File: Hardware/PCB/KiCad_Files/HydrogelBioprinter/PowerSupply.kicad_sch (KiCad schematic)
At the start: 11 parts, among them J3 Screw_Terminal_01x02, U4 AP3211KTR-G1

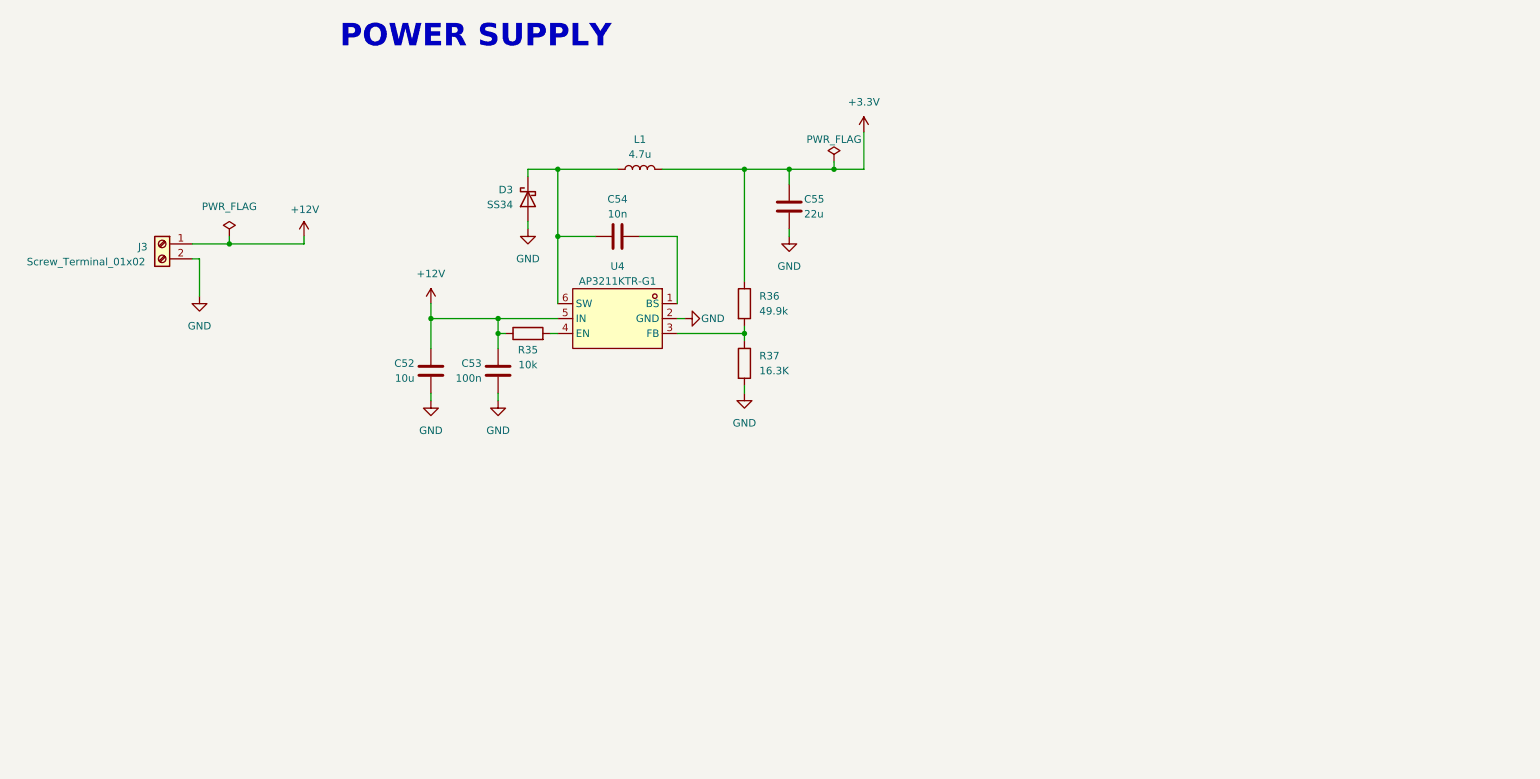
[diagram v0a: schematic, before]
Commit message: Schematic Update, PCB preliminary layout, Machine Design addition, and LaTeX report addition
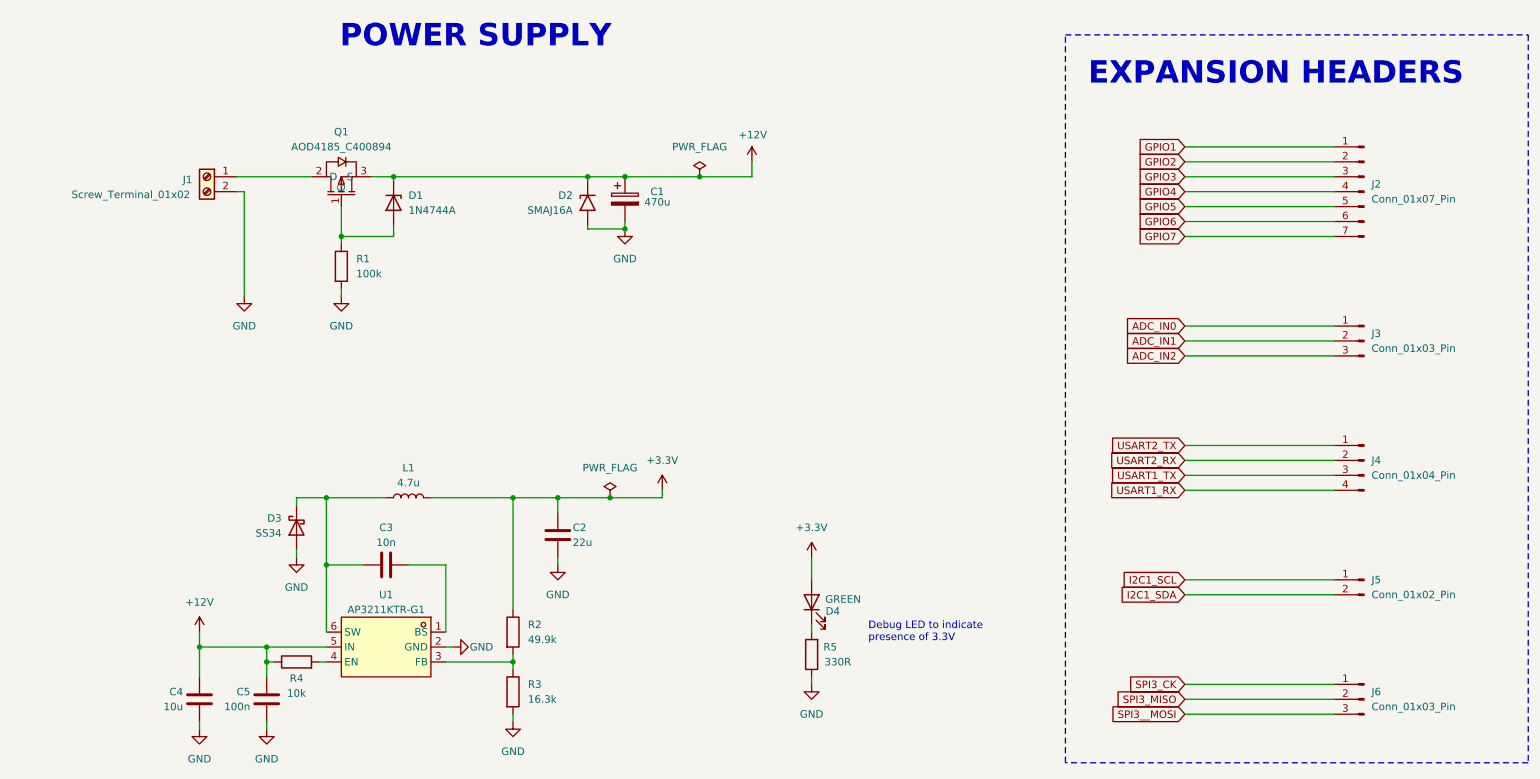
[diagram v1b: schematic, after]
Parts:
- added C1: 470u, Capacitor_THT:CP_Radial_D10.0mm_P5.00mm, symbol Device:C_Polarized
- added D1: 1N4744A, Diode_THT:D_DO-41_SOD81_P10.16mm_Horizontal, symbol Diode:1N47xxA
- added D2: SMAJ16A, Diode_SMD:D_SMA, symbol Diode:SMAJ16A
- added D4: GREEN, LED_SMD:LED_0805_2012Metric, symbol Device:LED
- added J2: Conn_01x07_Pin, Connector_PinHeader_2.54mm:PinHeader_1x07_P2.54mm_Vertical, symbol Connector:Conn_01x07_Pin
- added J3, J6: Conn_01x03_Pin, Connector_PinHeader_2.54mm:PinHeader_1x03_P2.54mm_Vertical, symbol Connector:Conn_01x03_Pin
- added J4: Conn_01x04_Pin, Connector_PinHeader_2.54mm:PinHeader_1x04_P2.54mm_Vertical, symbol Connector:Conn_01x04_Pin
- added J5: Conn_01x02_Pin, Connector_PinHeader_2.54mm:PinHeader_1x02_P2.54mm_Vertical, symbol Connector:Conn_01x02_Pin
- added Q1: AOD4185_C400894, AOD4185:TO-252-3_L6.6-W6.1-P4.57-LS9.9-BR-CW, symbol AOD4185:AOD4185_C400894
- added R1: 100k, Resistor_SMD:R_0805_2012Metric, symbol Device:R
- added R5: 330R, Resistor_THT:R_Axial_DIN0207_L6.3mm_D2.5mm_P10.16mm_Horizontal, symbol Device:R
- C2: renamed from C55; footprint (none) -> Capacitor_SMD:C_0805_2012Metric
- C3: renamed from C54; footprint (none) -> Capacitor_SMD:C_0603_1608Metric
- C4: renamed from C52; footprint (none) -> Capacitor_SMD:C_0805_2012Metric
- C5: renamed from C53; footprint (none) -> Capacitor_SMD:C_0603_1608Metric
- J1: renamed from J3; footprint (none) -> TerminalBlock_Phoenix:TerminalBlock_Phoenix_MKDS-1,5-2-5.08_1x02_P5.08mm_Horizontal
- L1: footprint (none) -> Inductor_SMD:L_7.3x7.3_H4.5
- R2: renamed from R36; footprint (none) -> Resistor_THT:R_Axial_DIN0207_L6.3mm_D2.5mm_P10.16mm_Horizontal
- R3: renamed from R37; value 16.3K -> 16.3k; footprint (none) -> Resistor_THT:R_Axial_DIN0207_L6.3mm_D2.5mm_P10.16mm_Horizontal
- R4: renamed from R35; footprint (none) -> Resistor_SMD:R_0805_2012Metric
- U1: renamed from U4; footprint easyeda2kicad:SOT-23-6_L2.9-W1.6-P0.95-LS2.8-BR -> AP3211KTR-G1:AP3211KTR-G1
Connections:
- net +12V: now also C1.1, D1.1 (K), D2.1 (A1), Q1.3 (S); no longer J1.1 (Pin_1)
- net +3.3V: now also D4.2 (A)
- net GND: now also C1.2, D2.2 (A2), R1.2, R5.1
- new net: D1.2 (A), Q1.1 (G), R1.1
- new net: J1.1 (Pin_1), Q1.2 (D)
- new net: D4.1 (K), R5.2
- new net ADC_IN0: J3.1 (Pin_1)
- new net ADC_IN1: J3.2 (Pin_2)
- new net ADC_IN2: J3.3 (Pin_3)
- new net GPIO1: J2.1 (Pin_1)
- new net GPIO2: J2.2 (Pin_2)
- new net GPIO3: J2.3 (Pin_3)
- new net GPIO4: J2.4 (Pin_4)
- new net GPIO5: J2.5 (Pin_5)
- new net GPIO6: J2.6 (Pin_6)
- new net GPIO7: J2.7 (Pin_7)
- new net I2C1_SCL: J5.1 (Pin_1)
- new net I2C1_SDA: J5.2 (Pin_2)
- new net SPI3_CK: J6.1 (Pin_1)
- new net SPI3_MISO: J6.2 (Pin_2)
- new net SPI3__MOSI: J6.3 (Pin_3)
- new net USART1_RX: J4.4 (Pin_4)
- new net USART1_TX: J4.3 (Pin_3)
- new net USART2_RX: J4.2 (Pin_2)
- new net USART2_TX: J4.1 (Pin_1)
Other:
- note added: "Debug LED to indicate presence of 3.3V"
- note added: "EXPANSION HEADERS"
- moved on the sheet: C2, C3, C4, C5, D3, J1, L1, R2, R3, R4, U1

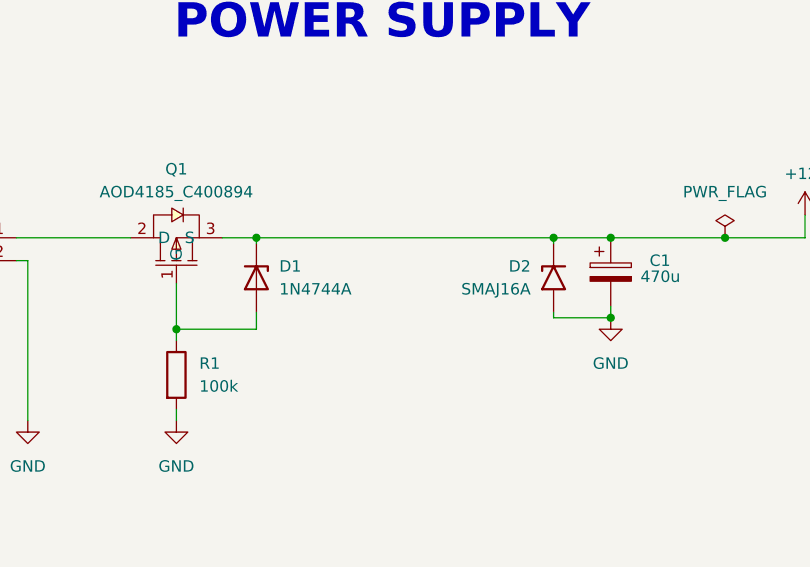
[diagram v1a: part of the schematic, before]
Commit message: Gantry Concept 1 Completion and PCB schematic update
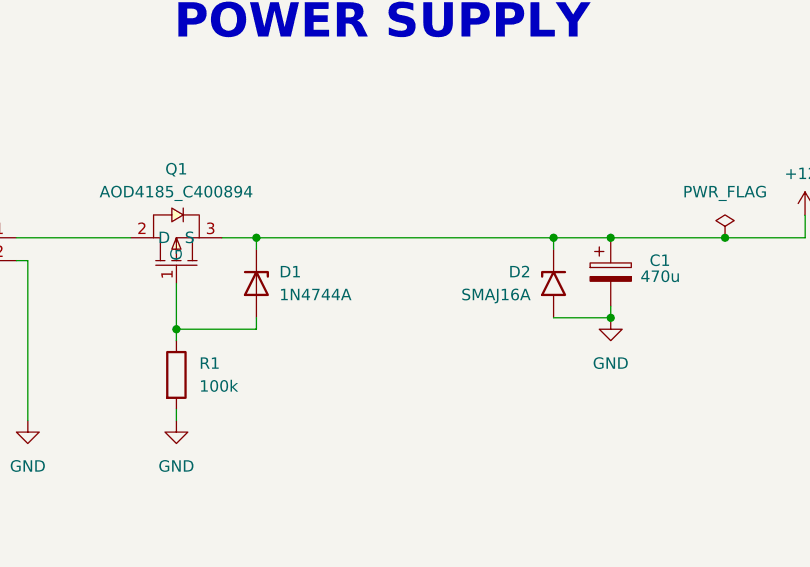
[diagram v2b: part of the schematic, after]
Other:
- moved on the sheet: D1, D2
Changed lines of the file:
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@@
 	)
 	(junction
+		(at 82.55 57.15)
+		(diameter 0)
+		(color 0 0 0 0)
+	)
+	(junction
 		(at 115.57 57.15)
 		(diameter 0)
@@
 		(color 0 0 0 0)
 	)
-	(junction
-		(at 82.55 57.15)
-		(diameter 0)
-		(color 0 0 0 0)
-	)
 	(wire
 		(pts
@@
 	(wire
 		(pts
-			(xy 115.57 57.785) (xy 115.57 57.15)
+			(xy 115.57 58.42) (xy 115.57 57.15)
 		)
 		(stroke
@@
 	(wire
 		(pts
-			(xy 82.55 65.405) (xy 82.55 67.31)
-		)
-		(stroke
-			(width 0)
-			(type default)
-		)
-	)
-	(wire
-		(pts
-			(xy 55.88 57.15) (xy 68.58 57.15)
+			(xy 82.55 66.04) (xy 82.55 67.31)
 		)
 		(stroke
@@
 	(wire
 		(pts
-			(xy 115.57 66.04) (xy 115.57 65.405)
-		)
-		(stroke
-			(width 0)
-			(type default)
-		)
-	)
-	(wire
-		(pts
 			(xy 121.92 64.77) (xy 121.92 66.04)
 		)
@@
 	(wire
 		(pts
+			(xy 73.66 62.23) (xy 73.66 67.31)
+		)
+		(stroke
+			(width 0)
+			(type default)
+		)
+	)
+	(wire
+		(pts
 			(xy 153.67 143.51) (xy 153.67 142.24)
 		)
@@
 	(wire
 		(pts
-			(xy 73.66 62.23) (xy 73.66 67.31)
-		)
-		(stroke
-			(width 0)
-			(type default)
-		)
-	)
-	(wire
-		(pts
 			(xy 217.17 62.23) (xy 242.57 62.23)
 		)
@@
 	(wire
 		(pts
-			(xy 60.96 139.7) (xy 60.96 137.16)
+			(xy 82.55 57.15) (xy 82.55 58.42)
 		)
 		(stroke
@@
 	(wire
 		(pts
-			(xy 143.51 57.15) (xy 143.51 54.61)
+			(xy 60.96 139.7) (xy 60.96 137.16)
 		)
 		(stroke
@@
 	(wire
 		(pts
-			(xy 82.55 57.785) (xy 82.55 57.15)
+			(xy 143.51 57.15) (xy 143.51 54.61)
 		)
 		(stroke
@@
 	(wire
 		(pts
+			(xy 55.88 57.15) (xy 68.58 57.15)
+		)
+		(stroke
+			(width 0)
+			(type default)
+		)
+	)
+	(wire
+		(pts
 			(xy 66.04 111.76) (xy 71.12 111.76)
 		)
@@
 	(symbol
 		(lib_id "Diode:1N47xxA")
-		(at 82.55 61.595 270)
+		(at 82.55 62.23 270)
 		(unit 1)
 		(exclude_from_sim no)
@@
 		(fields_autoplaced yes)
 		(property "Reference" "D1"
-			(at 85.09 60.3249 90)
+			(at 85.09 60.9599 90)
 			(effects
 				(font
@@
 		)
 		(property "Value" "1N4744A"
-			(at 85.09 62.8649 90)
+			(at 85.09 63.4999 90)
 			(effects
 				(font
@@
 		)
 		(property "Footprint" "Diode_THT:D_DO-41_SOD81_P10.16mm_Horizontal"
-			(at 78.105 61.595 0)
+			(at 78.105 62.23 0)
 			(effects
 				(font
@@
 		)
 		(property "Datasheet" "https://www.vishay.com/docs/85816/1n4728a.pdf"
-			(at 82.55 61.595 0)
+			(at 82.55 62.23 0)
 			(effects
 				(font
@@
 		)
 		(property "Description" "1300mW Silicon planar power Zener diodes, DO-41"
-			(at 82.55 61.595 0)
+			(at 82.55 62.23 0)
 			(effects
 				(font
@@
 	(symbol
 		(lib_id "Diode:SMAJ16A")
-		(at 115.57 61.595 90)
+		(at 115.57 62.23 90)
 		(mirror x)
 		(unit 1)
@@
 		(dnp no)
 		(property "Reference" "D2"
-			(at 113.03 60.3249 90)
+			(at 113.03 60.9599 90)
 			(effects
 				(font
@@
 		)
 		(property "Value" "SMAJ16A"
-			(at 113.03 62.8649 90)
+			(at 113.03 63.4999 90)
 			(effects
 				(font
@@
 		)
 		(property "Footprint" "Diode_SMD:D_SMA"
-			(at 120.65 61.595 0)
+			(at 120.65 62.23 0)
 			(effects
 				(font
@@
 		)
 		(property "Datasheet" "https://www.littelfuse.com/media?resourcetype=datasheets&itemid=75e32973-b177-4ee3-a0ff-cedaf1abdb93&filename=smaj-datasheet"
-			(at 115.57 60.325 0)
+			(at 115.57 60.96 0)
 			(effects
 				(font
@@
 		)
 		(property "Description" "400W unidirectional Transient Voltage Suppressor, 16.0Vr, SMA(DO-214AC)"
-			(at 115.57 61.595 0)
+			(at 115.57 62.23 0)
 			(effects
 				(font

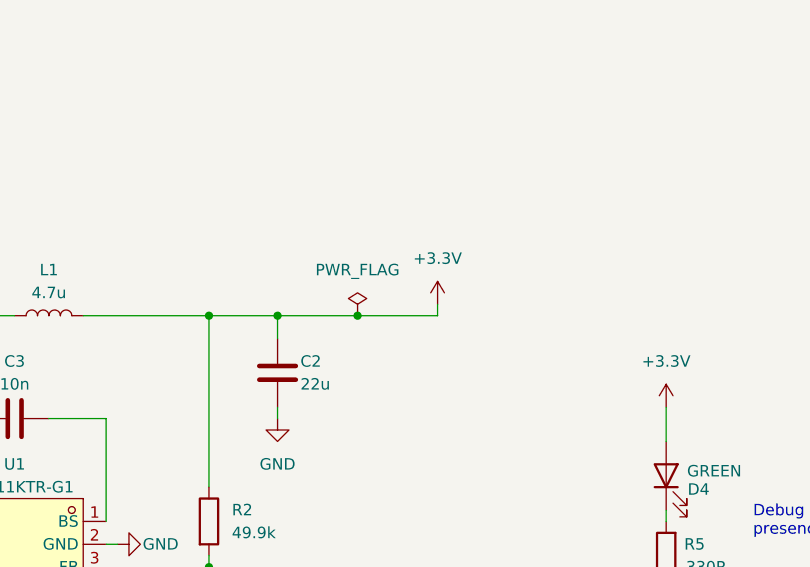
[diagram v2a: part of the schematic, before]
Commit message: PCB Catastrophe
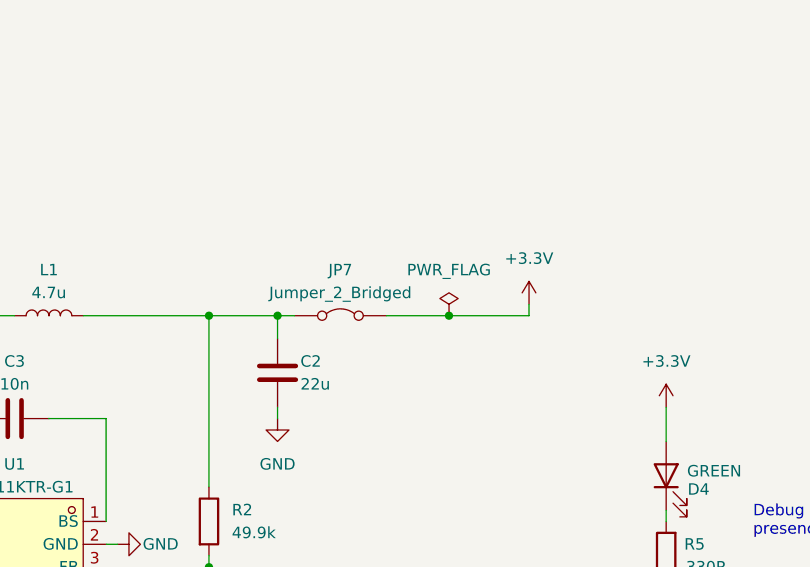
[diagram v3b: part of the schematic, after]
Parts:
- added JP7: Jumper_2_Bridged, TestPoint:TestPoint_2Pads_Pitch2.54mm_Drill0.8mm, symbol Jumper:Jumper_2_Bridged
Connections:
- net +3.3V: now also JP7.1 (A); no longer C2.1, L1.2, R2.1
- new net: C2.1, JP7.2 (B), L1.2, R2.1
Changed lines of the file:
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@@
 	)
 	(junction
+		(at 129.54 111.76)
+		(diameter 0)
+		(color 0 0 0 0)
+	)
+	(junction
 		(at 121.92 66.04)
 		(diameter 0)
@@
 	)
 	(junction
-		(at 119.38 111.76)
-		(diameter 0)
-		(color 0 0 0 0)
-	)
-	(junction
 		(at 73.66 67.31)
 		(diameter 0)
@@
 	(wire
 		(pts
+			(xy 138.43 110.49) (xy 138.43 111.76)
+		)
+		(stroke
+			(width 0)
+			(type default)
+		)
+	)
+	(wire
+		(pts
 			(xy 217.17 107.95) (xy 242.57 107.95)
 		)
@@
 	(wire
 		(pts
-			(xy 110.49 111.76) (xy 119.38 111.76)
+			(xy 110.49 111.76) (xy 112.395 111.76)
 		)
 		(stroke
@@
 	(wire
 		(pts
+			(xy 129.54 111.76) (xy 122.555 111.76)
+		)
+		(stroke
+			(width 0)
+			(type default)
+		)
+	)
+	(wire
+		(pts
 			(xy 82.55 66.04) (xy 82.55 67.31)
 		)
@@
 	(wire
 		(pts
-			(xy 119.38 111.76) (xy 128.27 111.76)
-		)
-		(stroke
-			(width 0)
-			(type default)
-		)
-	)
-	(wire
-		(pts
 			(xy 73.66 62.23) (xy 73.66 67.31)
 		)
@@
 	(wire
 		(pts
-			(xy 128.27 111.76) (xy 128.27 110.49)
-		)
-		(stroke
-			(width 0)
-			(type default)
-		)
-	)
-	(wire
-		(pts
 			(xy 60.96 139.7) (xy 60.96 142.24)
 		)
@@
 	(wire
 		(pts
+			(xy 129.54 111.76) (xy 138.43 111.76)
+		)
+		(stroke
+			(width 0)
+			(type default)
+		)
+	)
+	(wire
+		(pts
 			(xy 55.88 57.15) (xy 68.58 57.15)
 		)
@@
 	)
 	(symbol
+		(lib_id "Jumper:Jumper_2_Bridged")
+		(at 117.475 111.76 0)
+		(mirror y)
+		(unit 1)
+		(exclude_from_sim no)
+		(in_bom yes)
+		(on_board yes)
+		(dnp no)
+		(property "Reference" "JP7"
+			(at 117.475 106.68 0)
+			(effects
+				(font
+					(size 1.27 1.27)
+				)
+			)
+		)
+		(property "Value" "Jumper_2_Bridged"
+			(at 117.475 109.22 0)
+			(effects
+				(font
+					(size 1.27 1.27)
+				)
+			)
+		)
+		(property "Footprint" "TestPoint:TestPoint_2Pads_Pitch2.54mm_Drill0.8mm"
+			(at 117.475 111.76 0)
+			(effects
+				(font
+					(size 1.27 1.27)
+				)
+				(hide yes)
+			)
+		)
+		(property "Datasheet" "~"
+			(at 117.475 111.76 0)
+			(effects
+				(font
+					(size 1.27 1.27)
+				)
+				(hide yes)
+			)
+		)
+		(property "Description" "Jumper, 2-pole, closed/bridged"
+			(at 117.475 111.76 0)
+			(effects
+				(font
+					(size 1.27 1.27)
+				)
+				(hide yes)
+			)
+		)
+		(pin "2"
+		)
+		(pin "1"
+		)
+		(instances
+			(project ""
+				(path "/01596983-65d8-4ce5-b1db-2b179549cf8e/542eae74-acbf-46e1-b185-2c268e477aa1"
+					(reference "JP7")
+					(unit 1)
+				)
+			)
+		)
+	)
+	(symbol
 		(lib_id "power:+24V")
 		(at 143.51 54.61 0)
@@
 	)
 	(symbol
-		(lib_id "power:+3.3V")
-		(at 128.27 110.49 0)
-		(unit 1)
-		(exclude_from_sim no)
-		(in_bom yes)
-		(on_board yes)
-		(dnp no)
-		(fields_autoplaced yes)
-		(property "Reference" "#PWR05"
-			(at 128.27 114.3 0)
-			(effects
-				(font
-					(size 1.27 1.27)
-				)
-				(hide yes)
-			)
-		)
-		(property "Value" "+3.3V"
-			(at 128.27 105.41 0)
-			(effects
-				(font
-					(size 1.27 1.27)
-				)
-			)
-		)
-		(property "Footprint" ""
-			(at 128.27 110.49 0)
-			(effects
-				(font
-					(size 1.27 1.27)
-				)
-				(hide yes)
-			)
-		)
-		(property "Datasheet" ""
-			(at 128.27 110.49 0)
-			(effects
-				(font
-					(size 1.27 1.27)
-				)
-				(hide yes)
-			)
-		)
-		(property "Description" "Power symbol creates a global label with name \"+3.3V\""
-			(at 128.27 110.49 0)
-			(effects
-				(font
-					(size 1.27 1.27)
-				)
-				(hide yes)
-			)
-		)
-		(pin "1"
-		)
-		(instances
-			(project "HydrogelBioprinter"
-				(path "/01596983-65d8-4ce5-b1db-2b179549cf8e/542eae74-acbf-46e1-b185-2c268e477aa1"
-					(reference "#PWR05")
-					(unit 1)
-				)
-			)
-		)
-	)
-	(symbol
 		(lib_id "Device:R")
 		(at 153.67 138.43 180)
@@
 	)
 	(symbol
+		(lib_id "power:+3.3V")
+		(at 138.43 110.49 0)
+		(unit 1)
+		(exclude_from_sim no)
+		(in_bom yes)
+		(on_board yes)
+		(dnp no)
+		(fields_autoplaced yes)
+		(property "Reference" "#PWR023"
+			(at 138.43 114.3 0)
+			(effects
+				(font
+					(size 1.27 1.27)
+				)
+				(hide yes)
+			)
+		)
+		(property "Value" "+3.3V"
+			(at 138.43 105.41 0)
+			(effects
+				(font
+					(size 1.27 1.27)
+				)
+			)
+		)
+		(property "Footprint" ""
+			(at 138.43 110.49 0)
+			(effects
+				(font
+					(size 1.27 1.27)
+				)
+				(hide yes)
+			)
+		)
+		(property "Datasheet" ""
+			(at 138.43 110.49 0)
+			(effects
+				(font
+					(size 1.27 1.27)
+				)
+				(hide yes)
+			)
+		)
+		(property "Description" "Power symbol creates a global label with name \"+3.3V\""
+			(at 138.43 110.49 0)
+			(effects
+				(font
+					(size 1.27 1.27)
+				)
+				(hide yes)
+			)
+		)
+		(pin "1"
+		)
+		(instances
+			(project "HydrogelBioprinter"
+				(path "/01596983-65d8-4ce5-b1db-2b179549cf8e/542eae74-acbf-46e1-b185-2c268e477aa1"
+					(reference "#PWR023")
+					(unit 1)
+				)
+			)
+		)
+	)
+	(symbol
 		(lib_id "Device:C")
 		(at 81.28 123.19 90)
@@
 	(symbol
 		(lib_id "power:PWR_FLAG")
-		(at 119.38 111.76 0)
+		(at 129.54 111.76 0)
 		(unit 1)
 		(exclude_from_sim no)
@@
 		(fields_autoplaced yes)
 		(property "Reference" "#FLG02"
-			(at 119.38 109.855 0)
+			(at 129.54 109.855 0)
 			(effects
 				(font
@@
 		)
 		(property "Value" "PWR_FLAG"
-			(at 119.38 106.68 0)
+			(at 129.54 106.68 0)
 			(effects
 				(font
@@
 		)
 		(property "Footprint" ""
-			(at 119.38 111.76 0)
+			(at 129.54 111.76 0)
 			(effects
 				(font
@@
 		)
 		(property "Datasheet" "~"
-			(at 119.38 111.76 0)
+			(at 129.54 111.76 0)
 			(effects
 				(font
@@
 		)
 		(property "Description" "Special symbol for telling ERC where power comes from"
-			(at 119.38 111.76 0)
+			(at 129.54 111.76 0)
 			(effects
 				(font
